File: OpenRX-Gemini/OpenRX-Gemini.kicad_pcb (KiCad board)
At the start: 6 copper layers, 13.8 x 13.7 mm, 67 parts, among them T1 0900PC16J0042001E, T2 0900PC16J0042001E, U1 ESP32-C3FH4, U10 RFX2401C, U11 SKY13588-460LF, U2 TLV75533PDQNR, U3 TS2306A 240GF MSM 9_C2976675, U4 LR1121IMLTRT, U5 OW7EL89CENUYO3YLC-32M, U6 SKY13588-460LF, U7 RFX2401C, U8 OW7EL89CENUYO3YLC-32M, U9 LR1121IMLTRT, X1 CJ17-400001010B20

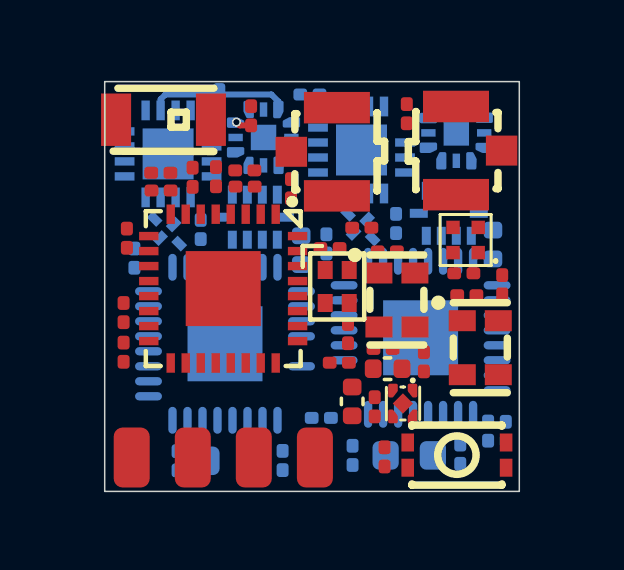
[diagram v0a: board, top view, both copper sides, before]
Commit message: initial routing for all
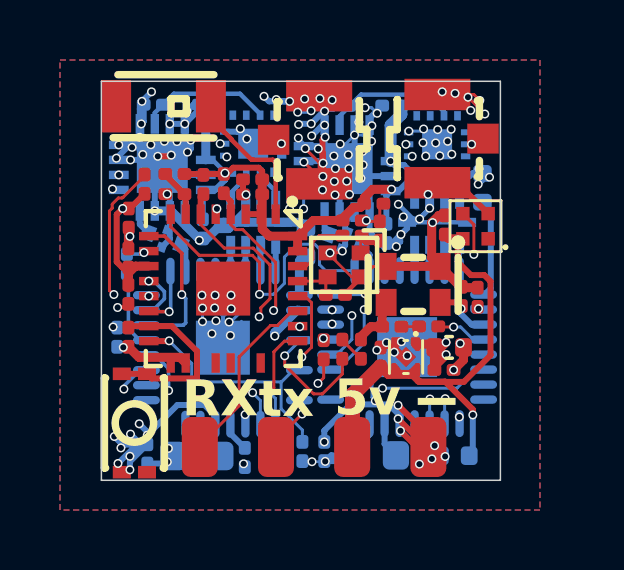
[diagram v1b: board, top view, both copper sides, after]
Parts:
- removed the C14 at (66.4, 45.9)
- removed the C15 at (64.7, 49.6)
- removed the C16 at (65.3, 45.3)
- removed the C17 at (74.3, 56.4)
- removed the C18 at (73.5, 51.1)
- removed the C20 at (68.0, 50.3)
- removed C21, C23: 100nF, Capacitor_SMD:C_0201_0603Metric
- removed the C22 at (67.4, 57.4)
- removed C30: 0.3pF, Capacitor_SMD:C_0201_0603Metric
- removed C31: 220pF, Capacitor_SMD:C_0201_0603Metric
- removed C32: 1uF, Capacitor_SMD:C_0201_0603Metric
- removed JP1, JP2: U.FL-R-SMT-1(80), OpenRX-Shared:RF-SMD_FRF05002-JSS103M
- removed the L1 at (65.7, 57.4)
- removed the R2 at (62.5, 50.6)
- removed the R7 at (74.9, 56.4)
- removed T1, T2: 0900PC16J0042001E, OpenRX-Shared:FILTER-SMD_10P-L2.0-W1.6-BL
- removed U10, U7: RFX2401C, OpenRX-Shared:QFN-16_L3.0-W3.0-P0.50-BL-EP1.7
- removed U11: SKY13588-460LF, OpenRX-Shared:QFN-12_L2.0-W2.0-P0.50-BL-EP0.8
- removed the U4 at (65.5, 53.5)
- removed U5, U8: OW7EL89CENUYO3YLC-32M, OpenRX-Shared:OSC-SMD_4P-L2.0-W1.6-BL_TXC_7Z
- removed the U6 at (66.8, 46.6)
- removed USB2, USB3: DEA102700LT-6307A2, OpenRX-Shared:FILTER-SMD_4P-L1.0-W0.5-L_DEA102700LT-XXX
- added C12: 100nF, Capacitor_SMD:C_0201_0603Metric, F.Cu at (72.8, 49.5)
- added C3: 100nF, Capacitor_SMD:C_0201_0603Metric, F.Cu at (70.5, 48.8)
- added C42: 0.3pF, Capacitor_SMD:C_0201_0603Metric, B.Cu at (63.1, 45.5)
- added C43: 220pF, Capacitor_SMD:C_0201_0603Metric, B.Cu at (64.8, 49.6)
- added C44: 1uF, Capacitor_SMD:C_0201_0603Metric, B.Cu at (65.0, 45.5)
- added C45: 0.3pF, Capacitor_SMD:C_0201_0603Metric, B.Cu at (69.3, 45.5)
- added C46: 220pF, Capacitor_SMD:C_0201_0603Metric, B.Cu at (70.9, 49.8)
- added C47: 1uF, Capacitor_SMD:C_0201_0603Metric, B.Cu at (71.1, 45.5)
- added C7: 100nF, Capacitor_SMD:C_0201_0603Metric, B.Cu at (66.2, 57.2)
- added C8: 10pF, Capacitor_SMD:C_0201_0603Metric, F.Cu at (69.4, 53.6)
- added C9: 4.7uF, Capacitor_SMD:C_0402_1005Metric, B.Cu at (68.2, 50.1)
- added FL4: 2450FM07D0034T, OpenRX-Shared:FILTER-SMD_4P-L1.0-W0.5-L, B.Cu at (63.5, 50.0)
- added FL5: 2450FM07D0034T, OpenRX-Shared:FILTER-SMD_4P-L1.0-W0.5-L, B.Cu at (69.5, 50.0)
- added JP4: U.FL-R-SMT-1(80), OpenRX-Shared:RF-SMD_FRF05002-JSS103M, F.Cu at (67.9, 46.7)
- added JP5: U.FL-R-SMT-1(80), OpenRX-Shared:RF-SMD_FRF05002-JSS103M, F.Cu at (73.3, 46.6)
- added L2: 10uH, Inductor_SMD:L_0603_1608Metric, B.Cu at (64.6, 57.2)
- added R10: 680R, Resistor_SMD:R_0201_0603Metric, F.Cu at (68.8, 53.7)
- added R11: 10k, Resistor_SMD:R_0201_0603Metric, F.Cu at (62.8, 48.1)
- added R3: 220R, Resistor_SMD:R_0201_0603Metric, F.Cu at (70.0, 53.6)
- added R5: 10k, Resistor_SMD:R_0201_0603Metric, B.Cu at (68.1, 57.0)
- added R9: 680R, Resistor_SMD:R_0201_0603Metric, B.Cu at (62.2, 50.8)
- added T4: 0900PC16J0042001E, OpenRX-Shared:FILTER-SMD_10P-L2.0-W1.6-BL, B.Cu at (66.4, 49.4)
- added T5: 0900PC16J0042001E, OpenRX-Shared:FILTER-SMD_10P-L2.0-W1.6-BL, B.Cu at (72.6, 49.4)
- added U1: OW7EL89CENUYO3YLC-32M, OpenRX-Shared:OSC-SMD_4P-L2.0-W1.6-BL_TXC_7Z, F.Cu at (71.8, 51.5)
- added U15: RFX2401C, OpenRX-Shared:QFN-16_L3.0-W3.0-P0.50-BL-EP1.7, B.Cu at (63.4, 47.6)
- added U16: SKY13414-485LF, OpenRX-Shared:QFN-14_L2.0-W2.0-P0.45-BL-EP, B.Cu at (66.4, 46.8)
- added U17: RFX2401C, OpenRX-Shared:QFN-16_L3.0-W3.0-P0.50-BL-EP1.7, B.Cu at (69.6, 47.6)
- added U18: SKY13414-485LF, OpenRX-Shared:QFN-14_L2.0-W2.0-P0.45-BL-EP, B.Cu at (72.6, 46.8)
- added U2: LR1121IMLTRT, OpenRX-Shared:QFN-32_L5.0-W5.0-P0.50-BL-EP3.7, B.Cu at (65.4, 53.6)
- C13: value 10pF -> 100nF; moved to B.Cu
- C14: renamed from C12; moved to B.Cu
- C24: moved to F.Cu
- C26: moved to B.Cu
- C27: value 100nF -> 10pF; moved to F.Cu
- R6: value 220R -> 10k; moved to B.Cu
- R8: value 10k -> 220R; moved to F.Cu
- moved C24 11.4 mm to (73.9, 51.9)
- moved U4 10.8 mm to (62.5, 56.1), turned to -90 degrees
- moved R7 9.43 mm to (62.3, 53.2), turned to 90 degrees
- moved R6 8.87 mm to (61.9, 53.2), turned to 90 degrees
- moved C13 7.09 mm to (62.9, 57.1), turned to -90 degrees
- moved TP4 5.83 mm to (72.3, 56.9)
- moved C26 5.56 mm to (72.0, 57.2), turned to 90 degrees
- moved C27 4.39 mm to (72.3, 52.9), turned to 0 degrees
- moved C14 3.87 mm to (73.2, 57.2), turned to 180 degrees
- moved R8 3.84 mm to (71.1, 52.9)
- moved C15 3.14 mm to (62.3, 50.6), turned to 90 degrees
- moved TP2 2.80 mm to (67.2, 56.9)
- moved C6 2.30 mm to (69.7, 49.4), turned to 0 degrees
- moved TP1 2.30 mm to (64.7, 56.9)
- moved C22 2.17 mm to (73.0, 53.6), turned to 0 degrees
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- renumbered C6 to C1, C1 to C10, C2 to C11, C3 to C15, C9 to C16, C4 to C17, C5 to C18, C8 to C2, C10 to C20, C11 to C22, C7 to C4, C19 to C6, L2 to L1, R4 to R2, R5 to R4, R3 to R7, U1 to U3, U3 to U4, U2 to U6
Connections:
- C13 pad 1: Net-(C13-Pad1) -> GND
- C13 pad 2: Net-(U4-XTA) -> +3V3
- C24 pad 1: GND -> +3V3
- C24 pad 2: +3V3 -> GND
- C25 pad 1: +3V3 -> GND
- C25 pad 2: GND -> /ESP32-C3 + 2x LR1121 Gemini/VTCXO
- C26 pad 2: Net-(U8-VDD) -> Net-(U9-VREG)
- C27 pad 1: GND -> Net-(C27-Pad1)
- C27 pad 2: Net-(U9-VREG) -> Net-(U9-XTA)
- R6 pad 1: Net-(C13-Pad1) -> +3V3
- R6 pad 2: Net-(U5-OUTPUT) -> /ESP32-C3 + 2x LR1121 Gemini/NSS2
- R8 pad 1: +3V3 -> Net-(C27-Pad1)
- R8 pad 2: /ESP32-C3 + 2x LR1121 Gemini/RST2 -> /ESP32-C3 + 2x LR1121 Gemini/XTA
- U9 pad 21: /ESP32-C3 + 2x LR1121 Gemini/MISO -> Net-(U9-DIO4)
- U9 pad 3: Net-(U8-VDD) -> /ESP32-C3 + 2x LR1121 Gemini/VTCXO
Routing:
- net GND: track 0.00 -> 155.9 mm, vias 0 -> 132
- net +3V3: track 0.54 -> 50.4 mm, vias 1 -> 14
- net +5V: track 0.00 -> 17.7 mm, vias 0 -> 1
- net /ESP32-C3 + 2x LR1121 Gemini/RST1: track 0.00 -> 14.5 mm, vias 0 -> 2
- net /ESP32-C3 + 2x LR1121 Gemini/DIO8-1: track 0.00 -> 14.2 mm, vias 0 -> 2
- net /ESP32-C3 + 2x LR1121 Gemini/DIO7-2: track 0.00 -> 13.0 mm, vias 0 -> 2
- net /ESP32-C3 + 2x LR1121 Gemini/IRQ1: track 0.00 -> 12.9 mm, vias 0 -> 2
- net /ESP32-C3 + 2x LR1121 Gemini/DIO8-2: track 0.00 -> 11.6 mm, vias 0 -> 2
- net /ESP32-C3 + 2x LR1121 Gemini/NSS1: track 0.00 -> 11.5 mm, vias 0 -> 2
- net /ESP32-C3 + 2x LR1121 Gemini/MOSI: track 0.00 -> 11.2 mm, vias 0 -> 2
- net /ESP32-C3 + 2x LR1121 Gemini/DIO7-1: track 0.00 -> 10.8 mm, vias 0 -> 2
- net /ESP32-C3 + 2x LR1121 Gemini/MISO: track 0.00 -> 10.6 mm, vias 0 -> 2
- net /ESP32-C3 + 2x LR1121 Gemini/RXEN2: track 0.00 -> 10.00 mm, vias 0 -> 2
- net /ESP32-C3 + 2x LR1121 Gemini/BUSY1: track 0.00 -> 9.98 mm, vias 0 -> 1
- net /ESP32-C3 + 2x LR1121 Gemini/BUSY2: track 0.00 -> 9.94 mm, vias 0 -> 2
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- added copper zone on In2.Cu, net +3V3
- added copper zone on B.Cu, net GND
- added copper zone on F.Cu, net GND
- added copper zone on In1.Cu, net GND
- added copper zone on In2.Cu, net GND
- added copper zone on In3.Cu, net GND
- added copper zone on In4.Cu, net GND
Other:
- board size 13.8 x 13.7 mm -> 13.3 x 13.3 mm
- board text added: "-"
- board text added: "5v"
- board text added: "RX"
- board text added: "tx"
